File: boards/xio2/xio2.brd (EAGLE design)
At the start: 170 x 100 mm, 376 parts, among them J1 12401598E4#2A, Q1 BSS138, Q2 BSS138, Q3 BC817-16LT3G, Q4 BC817-16LT3G, Y2 FA-238 25.0000MB-K3

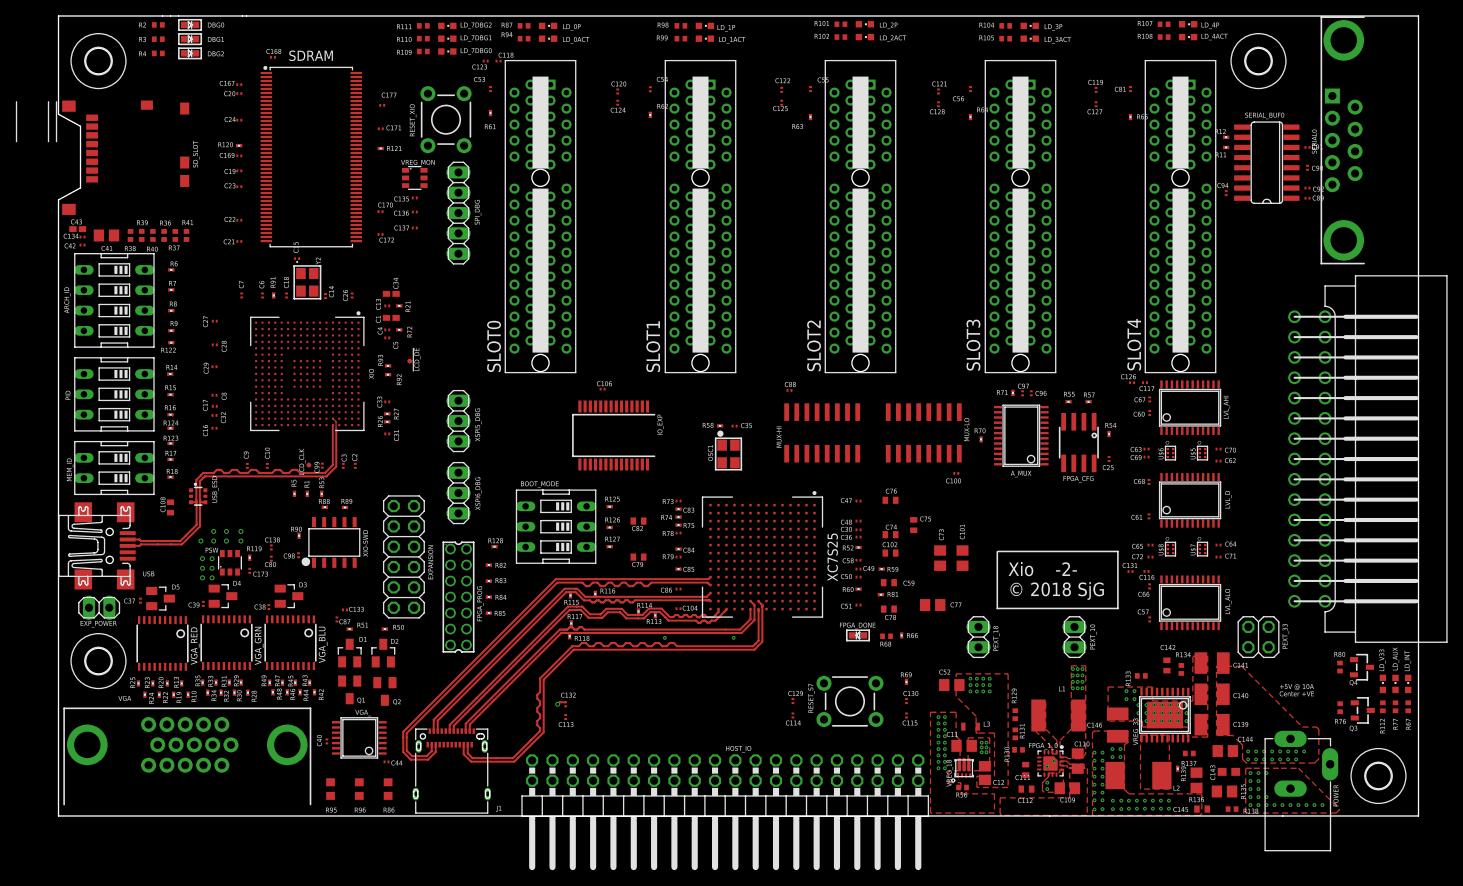
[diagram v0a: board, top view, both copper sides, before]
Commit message: routed board
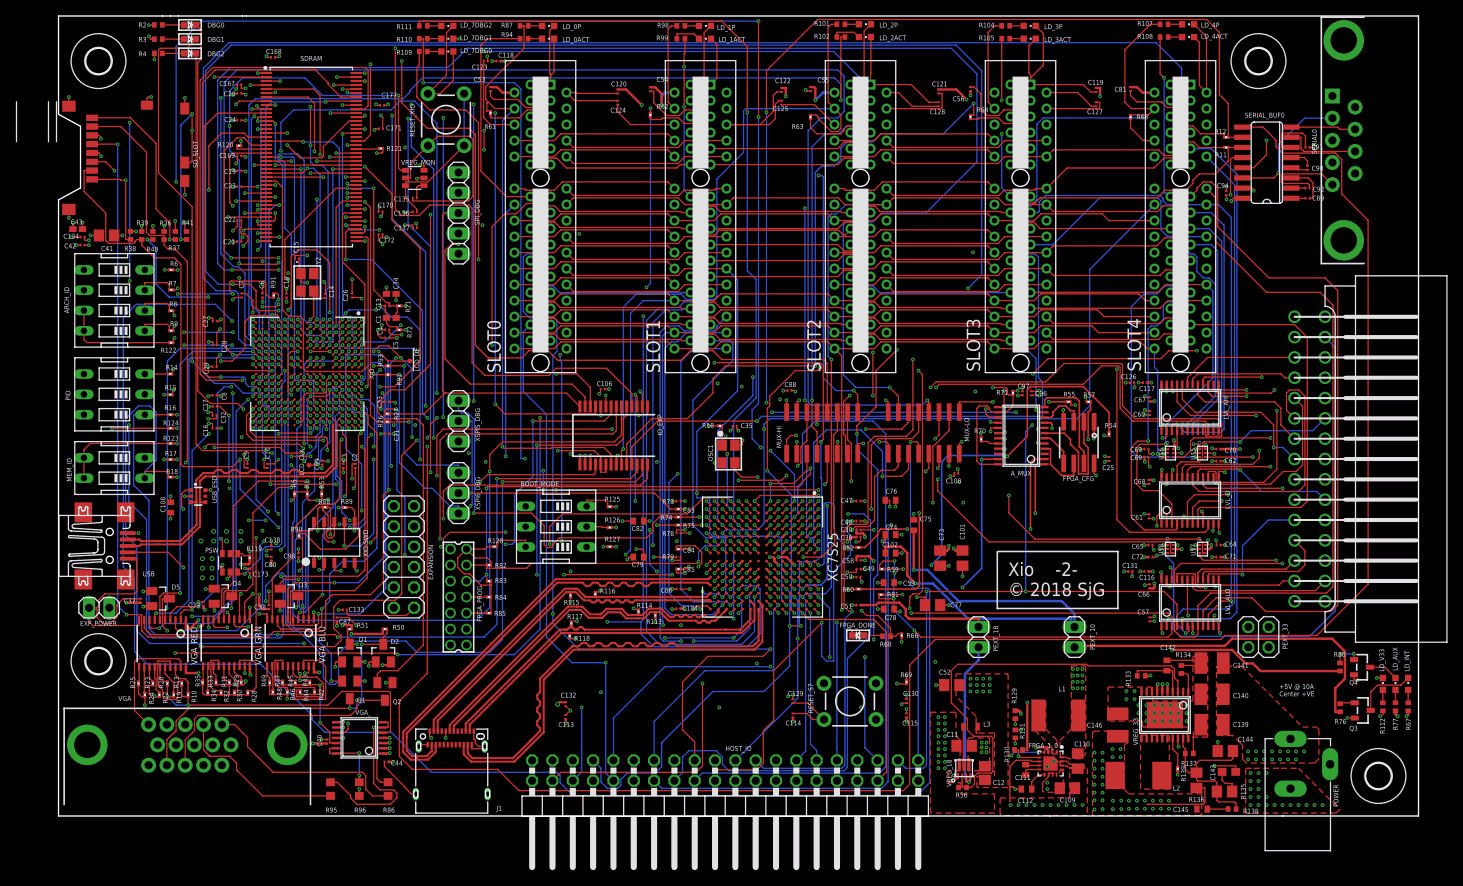
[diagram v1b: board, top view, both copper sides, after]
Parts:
- moved C99 0.40 mm to (33.0, 44.8)
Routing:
- net GND: track 0.00 -> 645.3 mm, vias 52 -> 362
- net HOST_A0: track 0.00 -> 405.4 mm, vias 0 -> 7
- net HOST_A11: track 0.00 -> 328.7 mm, vias 0 -> 7
- net HOST_A12: track 0.00 -> 318.0 mm, vias 0 -> 8
- net HOST_A2: track 0.00 -> 303.8 mm, vias 0 -> 6
- net HOST_A6: track 0.00 -> 303.2 mm, vias 0 -> 5
- net HOST_A7: track 0.00 -> 300.8 mm, vias 0 -> 5
- net HOST_A1: track 0.00 -> 294.3 mm, vias 0 -> 8
- net HOST_A9: track 0.00 -> 284.1 mm, vias 0 -> 9
- net HOST_A10: track 0.00 -> 280.2 mm, vias 0 -> 8
- net HOST_A5: track 0.00 -> 279.4 mm, vias 0 -> 4
- net HOST_A3: track 0.00 -> 278.3 mm, vias 0 -> 4
- net HOST_A4: track 0.00 -> 270.4 mm, vias 0 -> 5
- net MCU_CTS: track 0.00 -> 266.8 mm, vias 0 -> 3
- net HOST_A15: track 0.00 -> 265.1 mm, vias 0 -> 8
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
